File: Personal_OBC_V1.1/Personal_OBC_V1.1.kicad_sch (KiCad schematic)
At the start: 5 parts, among them U1 STM32F302K8Ux, U2 MS560702BA03-50, X1 ECS-2520MV-xxx-xx

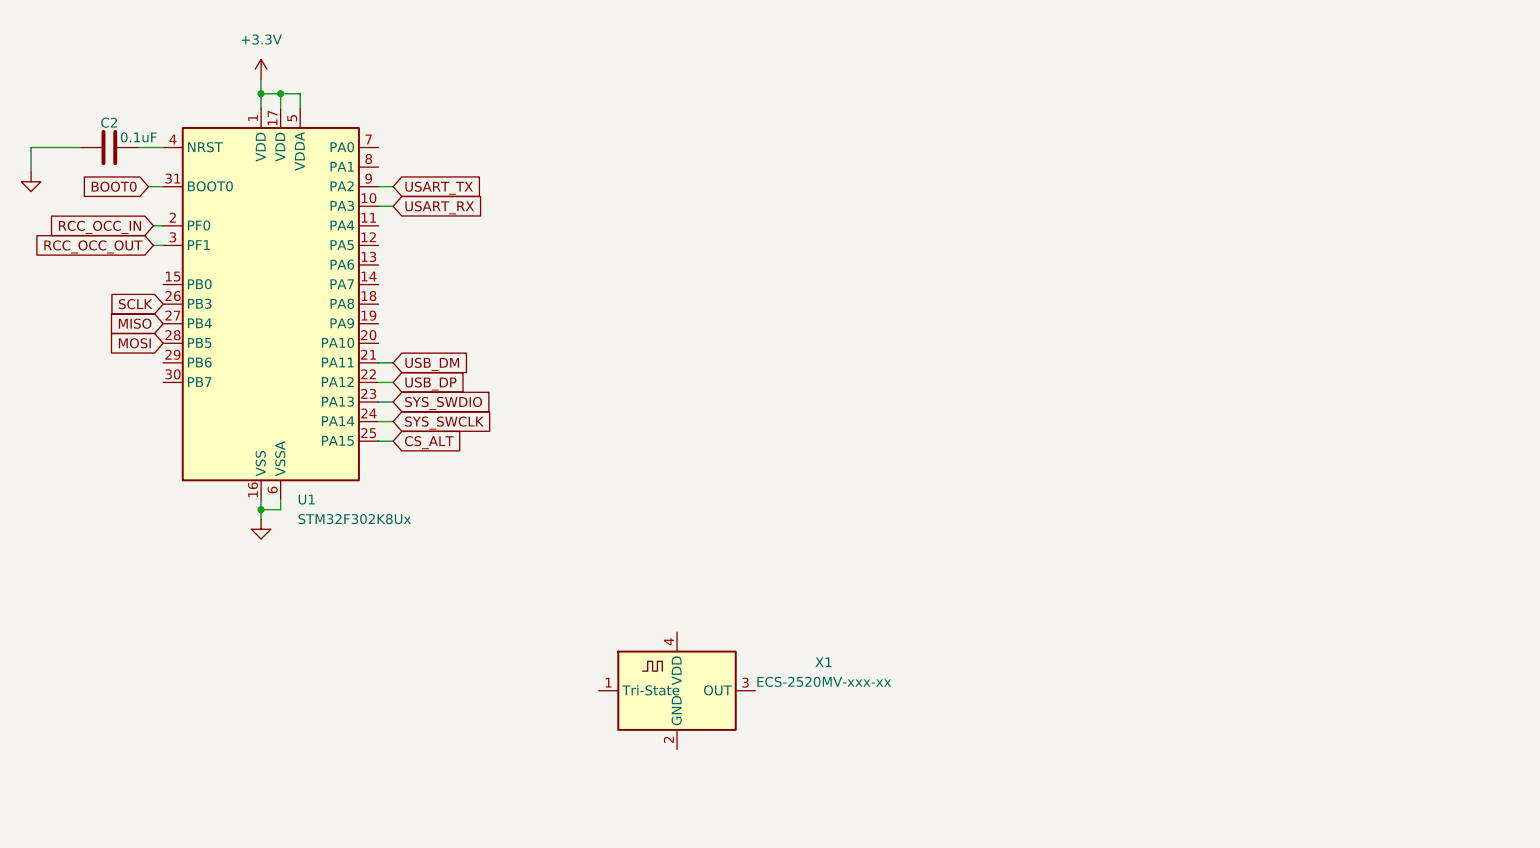
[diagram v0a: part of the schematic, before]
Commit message: A
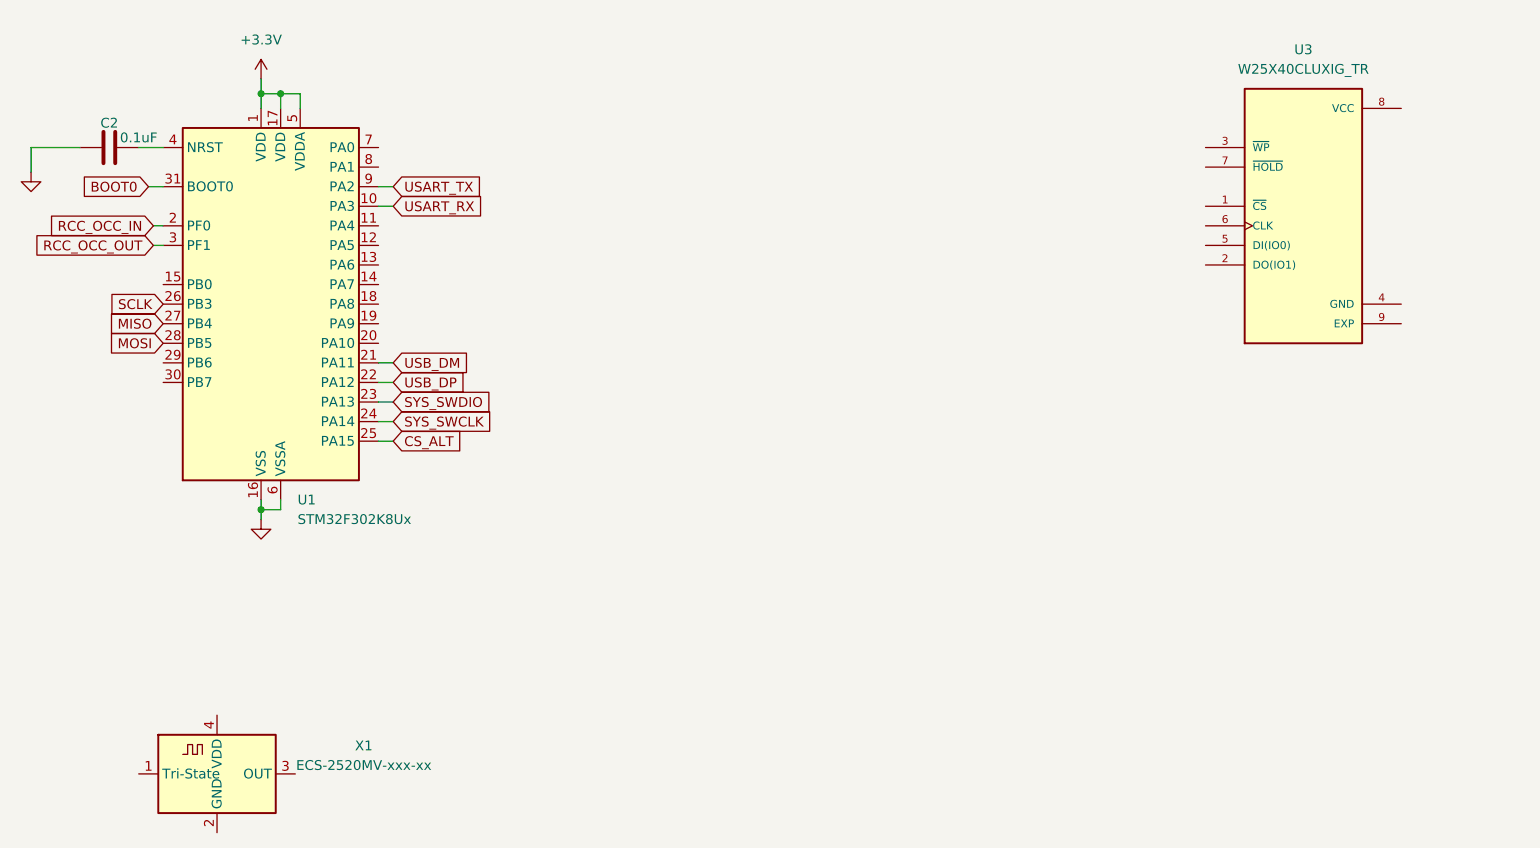
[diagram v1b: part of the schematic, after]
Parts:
- added U3: W25X40CLUXIG_TR, W25X40CLUXIG_TR:PSON50P300X200X60-9N, symbol W25X40CLUXIG TR:W25X40CLUXIG_TR
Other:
- moved on the sheet: X1
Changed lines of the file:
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@@
     )
   )
-  (symbol (lib_id "Oscillator:ECS-2520MV-xxx-xx") (at 99.06 99.695 0) (unit 1)
-    (in_bom yes) (on_board yes) (dnp no) (fields_autoplaced)
-    (property "Reference" "X1" (at 118.11 96.0471 0)
-      (effects (font (size 1.27 1.27)))
-    )
-    (property "Value" "ECS-2520MV-xxx-xx" (at 118.11 98.5871 0)
-      (effects (font (size 1.27 1.27)))
-    )
-    (property "Footprint" "Oscillator:Oscillator_SMD_ECS_2520MV-xxx-xx-4Pin_2.5x2.0mm" (at 110.49 108.585 0)
-      (effects (font (size 1.27 1.27)) hide)
-    )
-    (property "Datasheet" "https://www.ecsxtal.com/store/pdf/ECS-2520MV.pdf" (at 94.615 96.52 0)
+  (symbol (lib_id "Oscillator:ECS-2520MV-xxx-xx") (at 39.37 110.49 0) (unit 1)
+    (in_bom yes) (on_board yes) (dnp no) (fields_autoplaced)
+    (property "Reference" "X1" (at 58.42 106.8421 0)
+      (effects (font (size 1.27 1.27)))
+    )
+    (property "Value" "ECS-2520MV-xxx-xx" (at 58.42 109.3821 0)
+      (effects (font (size 1.27 1.27)))
+    )
+    (property "Footprint" "Oscillator:Oscillator_SMD_ECS_2520MV-xxx-xx-4Pin_2.5x2.0mm" (at 50.8 119.38 0)
+      (effects (font (size 1.27 1.27)) hide)
+    )
+    (property "Datasheet" "https://www.ecsxtal.com/store/pdf/ECS-2520MV.pdf" (at 34.925 107.315 0)
       (effects (font (size 1.27 1.27)) hide)
     )
@@
         )
       )
+    )
+  )
+  (symbol (lib_id "W25X40CLUXIG TR:W25X40CLUXIG_TR") (at 180.34 39.37 0) (unit 1)
+    (in_bom yes) (on_board yes) (dnp no) (fields_autoplaced)
+    (property "Reference" "U3" (at 180.34 16.51 0)
+      (effects (font (size 1.27 1.27)))
+    )
+    (property "Value" "W25X40CLUXIG_TR" (at 180.34 19.05 0)
+      (effects (font (size 1.27 1.27)))
+    )
+    (property "Footprint" "W25X40CLUXIG_TR:PSON50P300X200X60-9N" (at 180.34 39.37 0)
+      (effects (font (size 1.27 1.27)) (justify bottom) hide)
+    )
+    (property "Datasheet" "" (at 180.34 39.37 0)
+      (effects (font (size 1.27 1.27)) hide)
+    )
+    (property "MF" "Winbond Electronics" (at 180.34 39.37 0)
+      (effects (font (size 1.27 1.27)) (justify bottom) hide)
+    )
+    (property "Description" "\nFLASH Memory IC 4Mb (512K x 8) SPI 104 MHz 8-USON (2x3)\n" (at 180.34 39.37 0)
+      (effects (font (size 1.27 1.27)) (justify bottom) hide)
+    )
+    (property "Package" "UFDFN-8 Winbond" (at 180.34 39.37 0)
+      (effects (font (size 1.27 1.27)) (justify bottom) hide)
+    )
+    (property "Price" "None" (at 180.34 39.37 0)
+      (effects (font (size 1.27 1.27)) (justify bottom) hide)
+    )
+    (property "Check_prices" "https://www.snapeda.com/parts/W25X40CLUXIG%20TR/Winbond+Electronics/view-part/?ref=eda" (at 180.34 39.37 0)
+      (effects (font (size 1.27 1.27)) (justify bottom) hide)
+    )
+    (property "STANDARD" "IPC-7351B" (at 180.34 39.37 0)
+      (effects (font (size 1.27 1.27)) (justify bottom) hide)
+    )
+    (property "PARTREV" "F" (at 180.34 39.37 0)
+      (effects (font (size 1.27 1.27)) (justify bottom) hide)
+    )
+    (property "SnapEDA_Link" "https://www.snapeda.com/parts/W25X40CLUXIG%20TR/Winbond+Electronics/view-part/?ref=snap" (at 180.34 39.37 0)
+      (effects (font (size 1.27 1.27)) (justify bottom) hide)
+    )
+    (property "MP" "W25X40CLUXIG TR" (at 180.34 39.37 0)
+      (effects (font (size 1.27 1.27)) (justify bottom) hide)
+    )
+    (property "Purchase-URL" "https://www.snapeda.com/api/url_track_click_mouser/?unipart_id=424425&manufacturer=Winbond Electronics&part_name=W25X40CLUXIG TR&search_term=None" (at 180.34 39.37 0)
+      (effects (font (size 1.27 1.27)) (justify bottom) hide)
+    )
+    (property "Availability" "In Stock" (at 180.34 39.37 0)
+      (effects (font (size 1.27 1.27)) (justify bottom) hide)
+    )
+    (property "MANUFACTURER" "Winbond" (at 180.34 39.37 0)
+      (effects (font (size 1.27 1.27)) (justify bottom) hide)
+    )
+    (pin "1")
+    (pin "2")
+    (pin "3")
+    (pin "4")
+    (pin "5")
+    (pin "6")
+    (pin "7")
+    (pin "8")
+    (pin "9")
+    (instances
+      (project "Personal_OBC_V1.1"
+        (path "/7aafcae6-20fd-4029-823b-72b16b42b1cc"
+          (reference "U3") (unit 1)
+        )
+      )

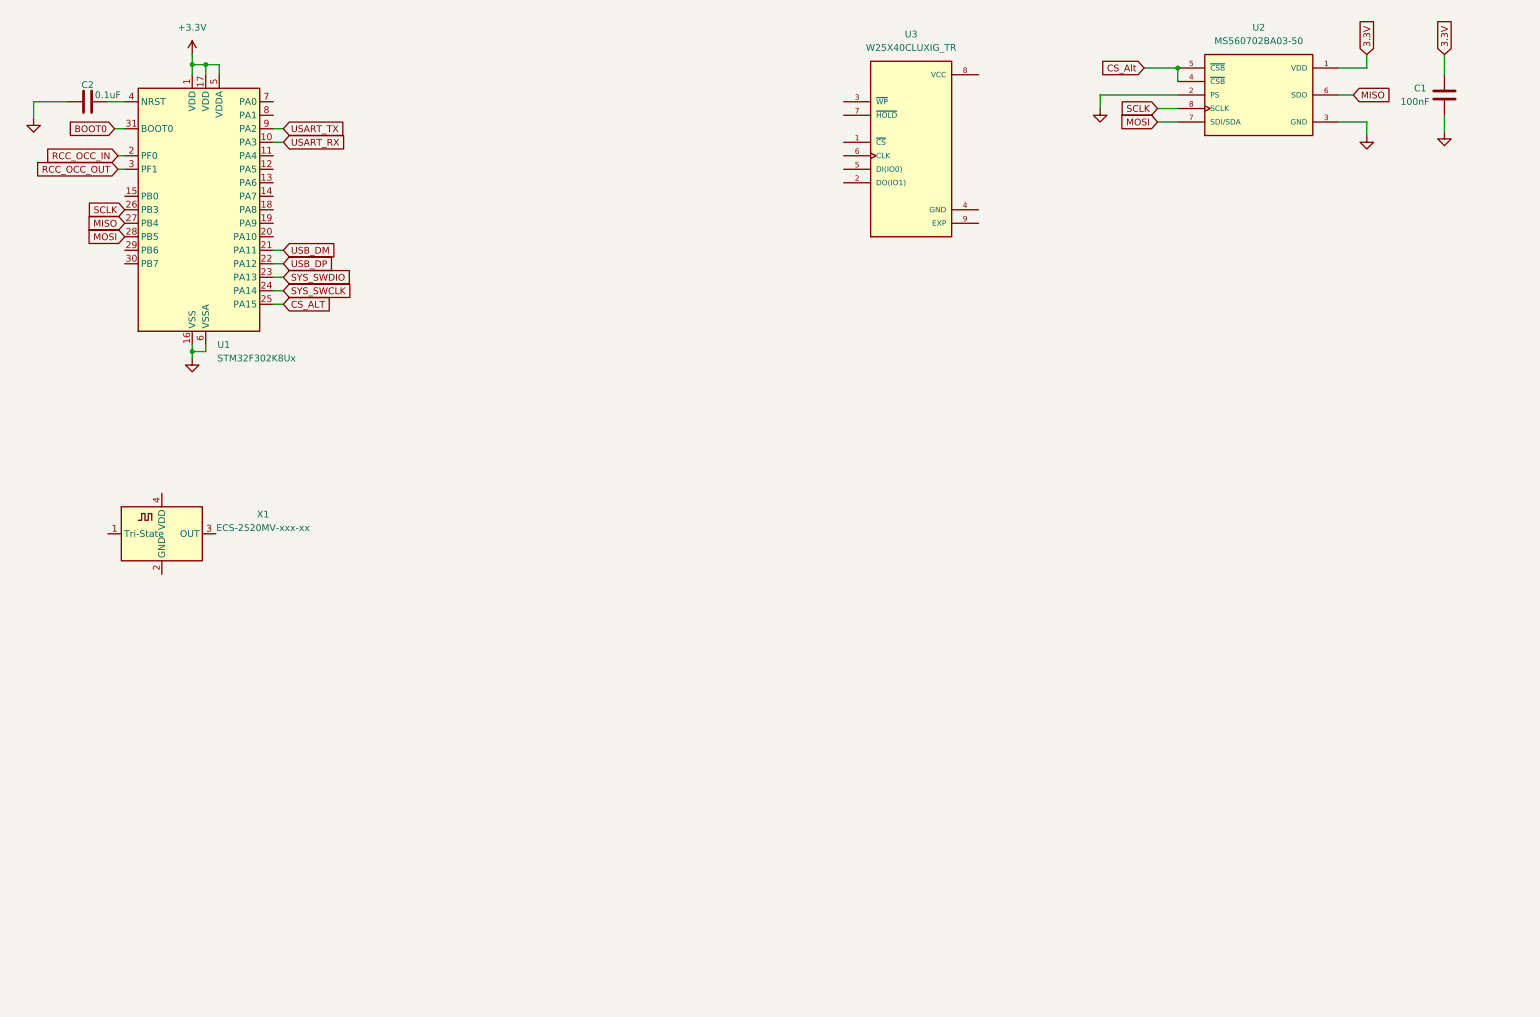
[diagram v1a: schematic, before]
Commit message: Personal Work
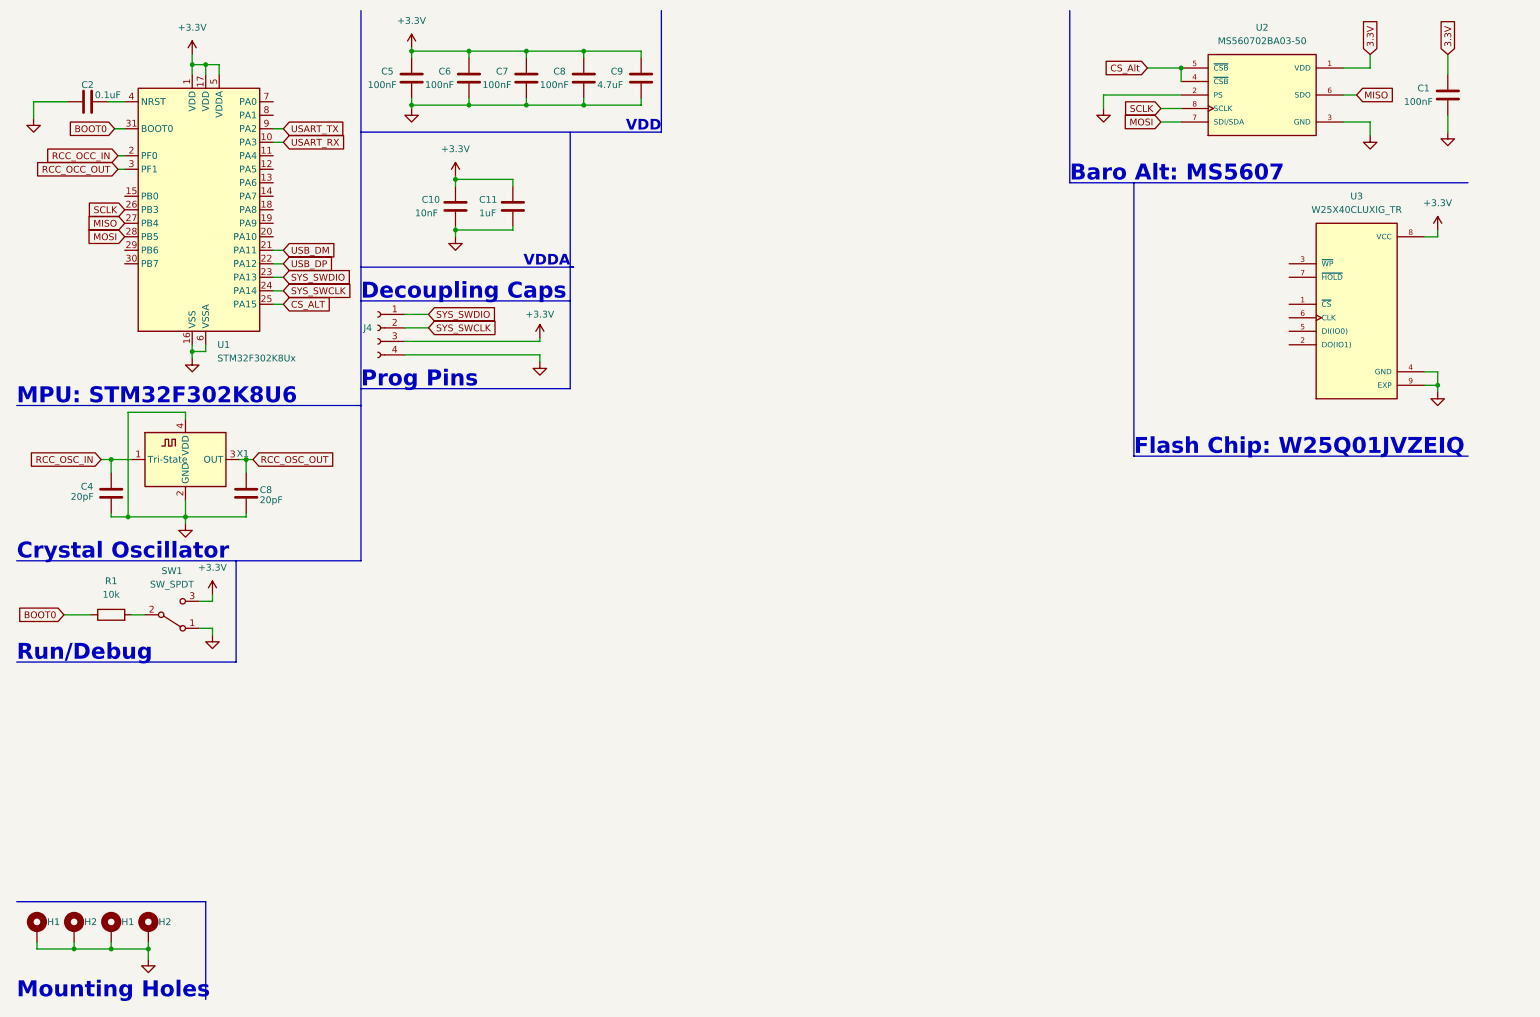
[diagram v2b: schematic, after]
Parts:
- added C10: 10nF, Capacitor_SMD:C_0402_1005Metric, symbol Device:C
- added C11: 1uF, Capacitor_SMD:C_0402_1005Metric, symbol Device:C
- added C4, C8: 20pF, Capacitor_SMD:C_0402_1005Metric, symbol Device:C
- added C5, C6, C7, C8: 100nF, Capacitor_SMD:C_0402_1005Metric, symbol Device:C
- added C9: 4.7uF, Capacitor_SMD:C_0402_1005Metric, symbol Device:C
- added H1 (x2), H2 (x2): MountingHole_Pad, MountingHole:MountingHole_3.2mm_M3_Pad_TopBottom, symbol Mechanical:MountingHole_Pad
- added J4: Conn_01x04_Socket, Connector_PinHeader_2.54mm:PinHeader_1x04_P2.54mm_Vertical, symbol Connector:Conn_01x04_Socket
- added R1: 10k, Resistor_SMD:R_0402_1005Metric, symbol Device:R
- added SW1: SW_SPDT, Jumper:SolderJumper-3_P1.3mm_Open_RoundedPad1.0x1.5mm_NumberLabels, symbol Switch:SW_SPDT
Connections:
- net +3.3V: now also U3.8 (VCC), C10.1, C11.1, C5.1, C6.1, C7.1, C8.1, C9.1, J4.3 (Pin_3), SW1.3 (C)
- net BOOT0: now also R1.1
- net GND: now also U3.4 (GND), U3.9 (EXP), X1.2 (GND), X1.4 (VDD), C10.2, C11.2, C4.2, C5.2, C6.2, C7.2, C8.2, C8.2, C9.2, H1.1, H1.1, H2.1, H2.1, J4.4 (Pin_4), SW1.1 (A)
- net SYS_SWCLK: now also J4.2 (Pin_2)
- net SYS_SWDIO: now also J4.1 (Pin_1)
- net RCC_OSC_IN: now reaches X1.1 (Tri-State)
- net RCC_OSC_IN: now also C4.1
- net RCC_OSC_OUT: now reaches X1.3 (OUT)
- net RCC_OSC_OUT: now also C8.1
- new net: R1.2, SW1.2 (B)
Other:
- note added: "Baro Alt: MS5607"
- note added: "Crystal Oscillator"
- note added: "Decoupling Caps"
- note added: "Flash Chip: W25Q01JVZEIQ"
- note added: "MPU: STM32F302K8U6"
- note added: "Mounting Holes"
- note added: "Prog Pins"
- note added: "Run/Debug"
- note added: "VDD"
- note added: "VDDA"
- moved on the sheet: C1, U2, U3, X1

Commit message: Personal Altimeter
Needs Radio Part
Needs Pyro Channels
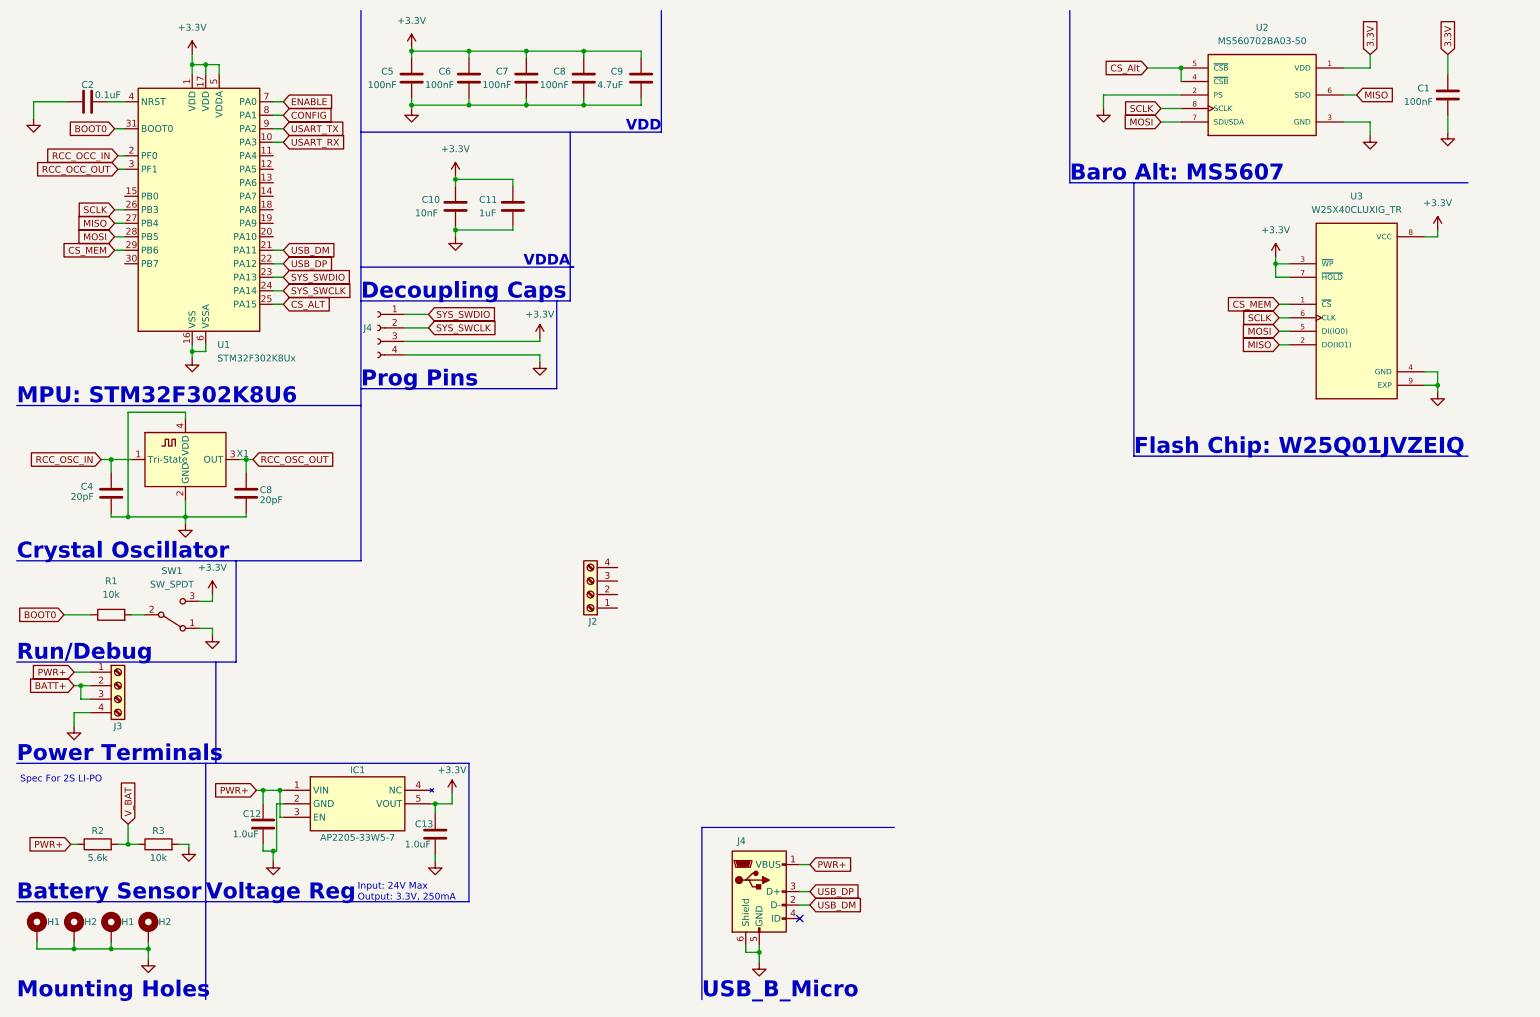
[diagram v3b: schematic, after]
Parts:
- added C12, C13: 1.0uF, symbol Device:C
- added IC1: AP2205-33W5-7, AP2205-33W5-7:SOT95P282X130-5N, symbol AP2205-33W5-7:AP2205-33W5-7
- added J2: PYRO CHANNELS, symbol Connector:Screw_Terminal_01x04
- added J3: POWER IN, symbol Connector:Screw_Terminal_01x04
- added J4: USB_B_Micro, Connector_USB:USB_Micro-B_Amphenol_10104110_Horizontal, symbol Connector:USB_B_Micro
- added R2: 5.6k, symbol Device:R
- added R3: 10k, symbol Device:R
- J4: value Conn_01x04_Socket -> PROG PINS
- U2: footprint MS5607:SON125P300X500X100-8N -> MS560702BA03-50:SON125P300X500X100-8N
- U3: footprint W25X40CLUXIG_TR:PSON50P300X200X60-9N -> W25X40CLUXIG TR:PSON50P300X200X60-9N
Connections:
- net +3.3V: now also U3.3 (~{WP}), U3.7 (~{HOLD}), C13.1, IC1.5 (VOUT)
- net GND: now also C12.2, C13.2, IC1.2 (GND), J3.4 (Pin_4), J4.5 (GND), J4.6 (Shield), R3.2
- net MISO: now also U3.2 (DO(IO1))
- net MOSI: now also U3.5 (DI(IO0))
- net SCLK: now also U3.6 (CLK)
- net USB_DM: now also J4.2 (D-)
- net USB_DP: now also J4.3 (D+)
- net CS_MEM: now reaches U1.29 (PB6)
- net CS_MEM: now also U3.1 (~{CS})
- net ENABLE: now reaches U1.7 (PA0)
- net CONFIG: now reaches U1.8 (PA1)
- new net BATT+: J3.2 (Pin_2), J3.3 (Pin_3)
- new net PWR+: C12.1, IC1.1 (VIN), IC1.3 (EN), J3.1 (Pin_1), J4.1 (VBUS), R2.1
- new net V_BAT: R2.2, R3.1
- no-connect marks 0 -> 1
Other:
- note added: "Battery Sensor"
- note added: "Input: 24V Max Output: 3.3V, 250mA"
- note added: "Power Terminals"
- note added: "Spec For 2S LI-PO"
- note added: "USB_B_Micro"
- note added: "Voltage Reg"
